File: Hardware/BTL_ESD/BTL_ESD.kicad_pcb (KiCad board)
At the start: 2 copper layers, 73.4 x 95.8 mm, 146 parts, among them J1 DC-005-5A-2.0, J2 BOOT, J3 Load Program, J4 Socket_TFT_1, J5 Socket_TFT_2, J6 USB_B_Micro, J7 220VAC, K1 SRD-05VDC-SL-C, Q1 MMBT2222A, Q2 MMBT2222A, Q3 MMBT2222A, Q4 MMBT2222A, SW1 MS-22D18G2ROHS, SW2 RESET, SW3 ENABLE, SW4 FLASH, U1 ICL7662CBA-T, U2 AMS1117-3.3, U3 TPS54331D, U4 STM32F103RCTx, U5 ESP32-WROOM-32E__4MB_HIGH_TEM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, U6 MCP6002-E_SN, U7 INA128UA, U8 CH340C, U9 PC817, Y1 8MHz, Y2 32.768KHz

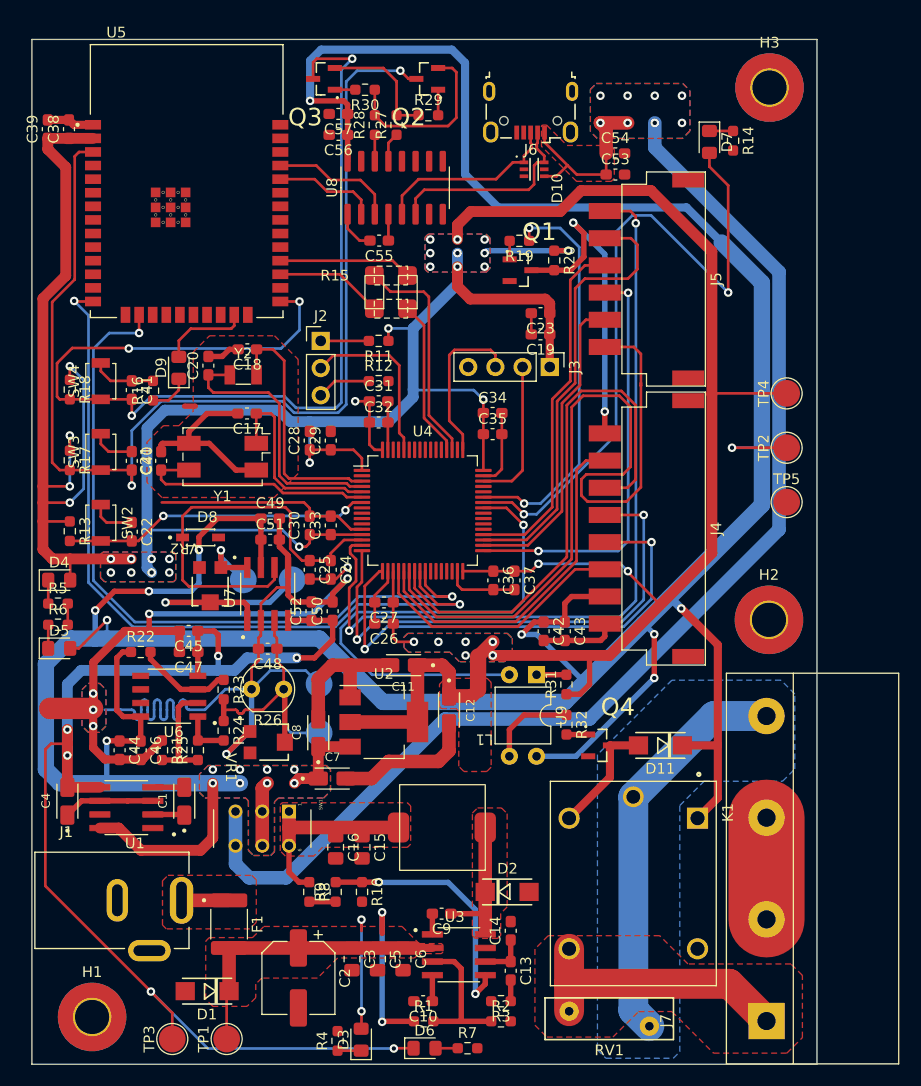
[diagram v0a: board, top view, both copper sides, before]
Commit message: update
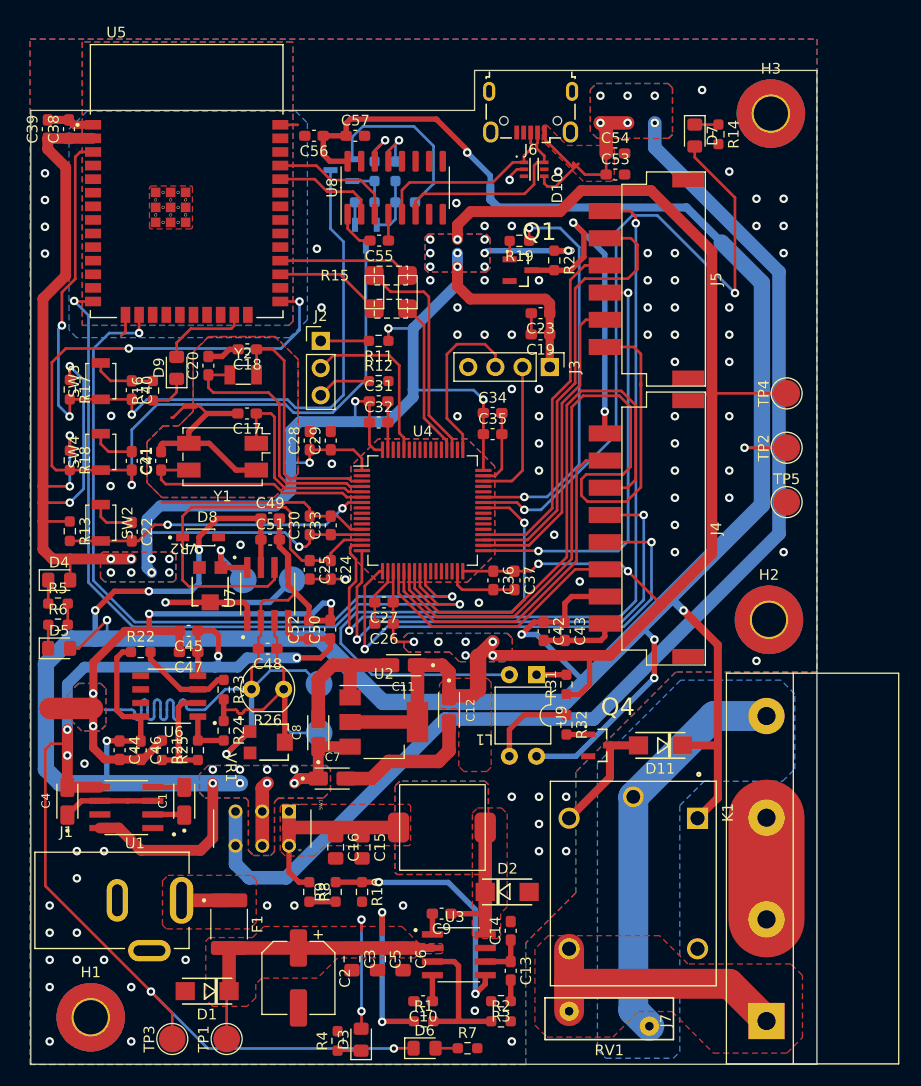
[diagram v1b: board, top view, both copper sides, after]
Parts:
- Q2, Q3, R27, R28, R29, R30: moved to B.Cu
- moved Q3 15.2 mm to (184.5, 59.3), turned to -90 degrees
- moved Q2 11.7 mm to (182.2, 53.2)
- moved R30 10.5 mm to (184.4, 56.2)
- moved R29 8.41 mm to (188.2, 56.2)
- moved C40 6.61 mm to (162.6, 73.8)
- moved C41 6.61 mm to (162.6, 80.4)
- moved R17 6.61 mm to (156.8, 73.7)
- moved R18 6.61 mm to (156.8, 80.3)
- moved SW3 6.61 mm to (159.7, 72.9)
- moved SW4 6.61 mm to (159.7, 79.5)
- moved R27 4.32 mm to (187.2, 53.3), turned to -90 degrees
- moved R28 4.32 mm to (185.3, 53.3), turned to -90 degrees
- moved C57 2.59 mm to (183.5, 50.0), turned to 0 degrees
- moved H3 2.44 mm to (222.3, 47.9)
- moved C56 2.28 mm to (179.6, 50.0)
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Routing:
- net EN: track 105.1 -> 78.7 mm, vias 2 -> 3
- net +5V: track 354.8 -> 336.2 mm
- net Net-(Q2-Pad1): track 2.38 -> 16.8 mm
- net RTS: track 16.9 -> 4.07 mm
- net FLASH: track 99.1 -> 89.6 mm, vias 4 -> 3
- net GND: track 117.6 -> 124.3 mm, vias 1 -> 88
- net DIR: track 11.5 -> 5.53 mm
- net GNDA: track 122.3 -> 116.8 mm, vias 6 -> 5
- net V_USB: track 130.6 -> 133.6 mm, vias 8 -> 6
- net +3V3: track 370.1 -> 367.4 mm
- net Net-(U8-~{RTS}): track 2.47 -> 4.75 mm, vias 0 -> 1
- net /STM32/LED_TEST: track 62.8 -> 64.6 mm
- net Net-(U8-~{DTR}): track 2.79 -> 4.56 mm, vias 0 -> 1
- net GND1: track 20.0 -> 21.4 mm
- net /STM32/SWCLK: track 15.2 -> 16.0 mm
- added copper zone on B.Cu, net GND
- added copper zone on F.Cu, net GND
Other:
- board size 73.4 x 95.8 mm -> 73.5 x 92.9 mm
